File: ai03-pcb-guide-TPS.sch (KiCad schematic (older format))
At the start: 24 parts, among them SW1 SW_Push, U1 ATmega32U4-AU, Y1 16MHz

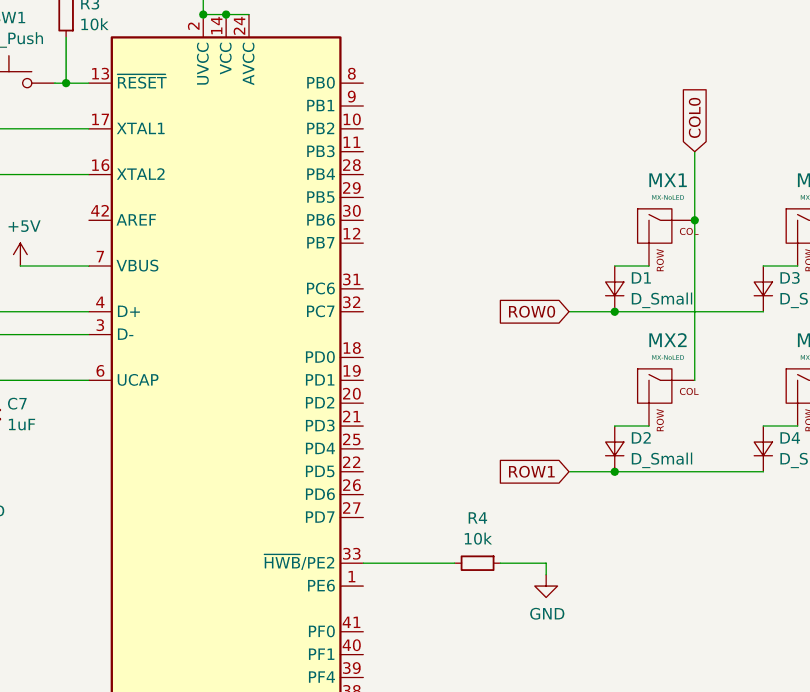
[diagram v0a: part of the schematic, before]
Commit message: Project Save
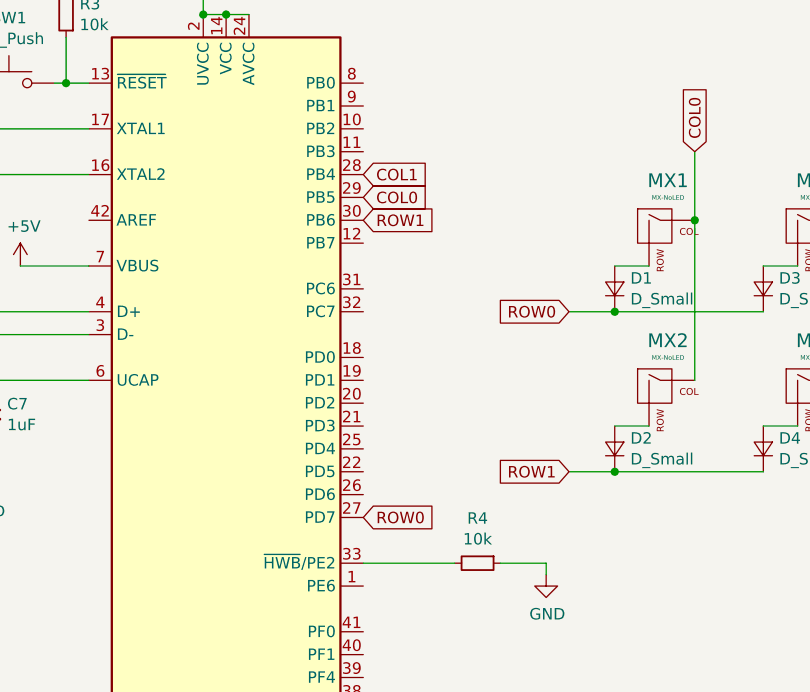
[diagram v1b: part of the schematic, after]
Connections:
- net COL0: now also U1.29 (PB5)
- net COL1: now also U1.28 (PB4)
- net ROW0: now also U1.27 (PD7)
- net ROW1: now also U1.30 (PB6)
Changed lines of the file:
@@
 Text GLabel 6750 2550 1    50   Input ~ 0
 COL1
+Text GLabel 4650 2650 2    50   Input ~ 0
+COL1
+Text GLabel 4650 2750 2    50   Input ~ 0
+COL0
+Text GLabel 4650 2850 2    50   Input ~ 0
+ROW1
+Text GLabel 4650 4150 2    50   Input ~ 0
+ROW0
 $EndSCHEMATC
